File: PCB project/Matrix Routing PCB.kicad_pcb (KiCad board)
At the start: 2 copper layers, 80 x 50.6 mm, 10 parts, among them J1 53261-0471, J2 JST_PH_S4B-PH-SM4-TB, J3 ESQ-105-23-T-D, J4 TSM-102-01-L-DH-A, J5 USB-A-S-X-X-SM2-R, U1 FT232RL

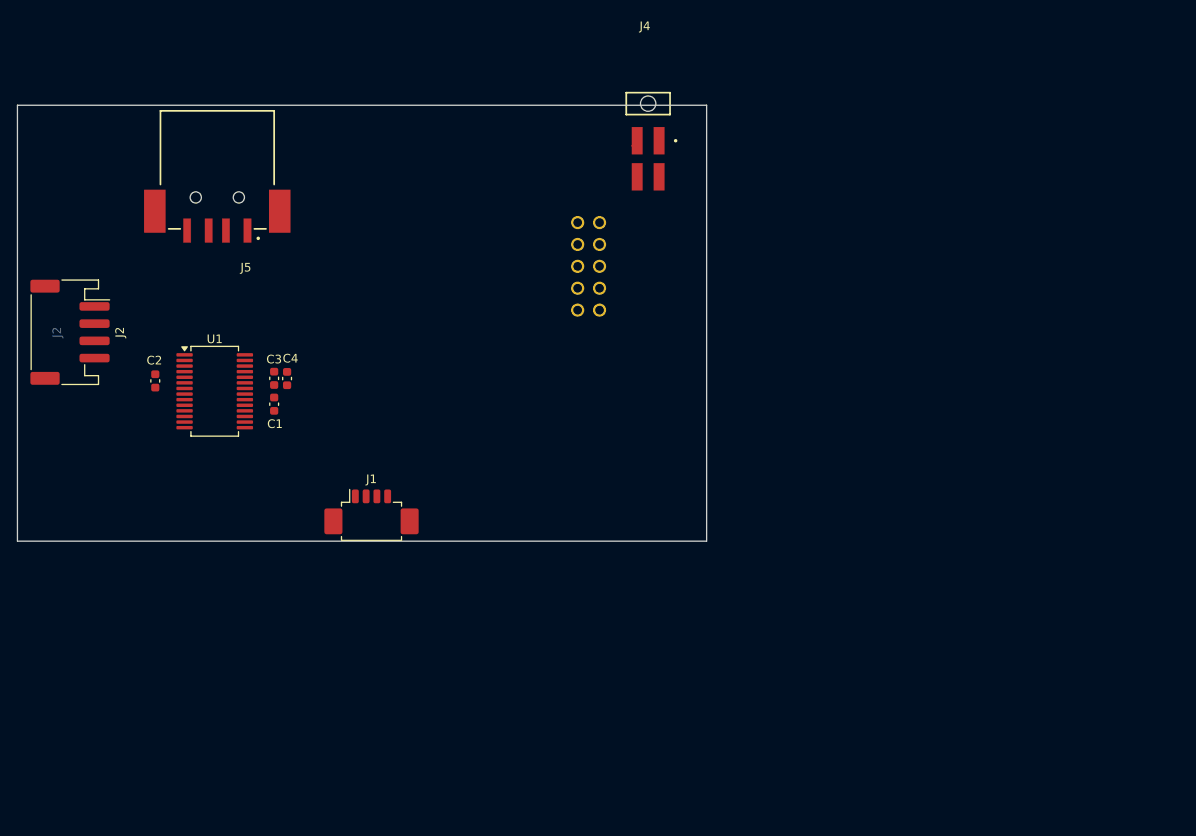
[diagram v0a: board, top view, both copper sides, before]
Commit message: Placement to review
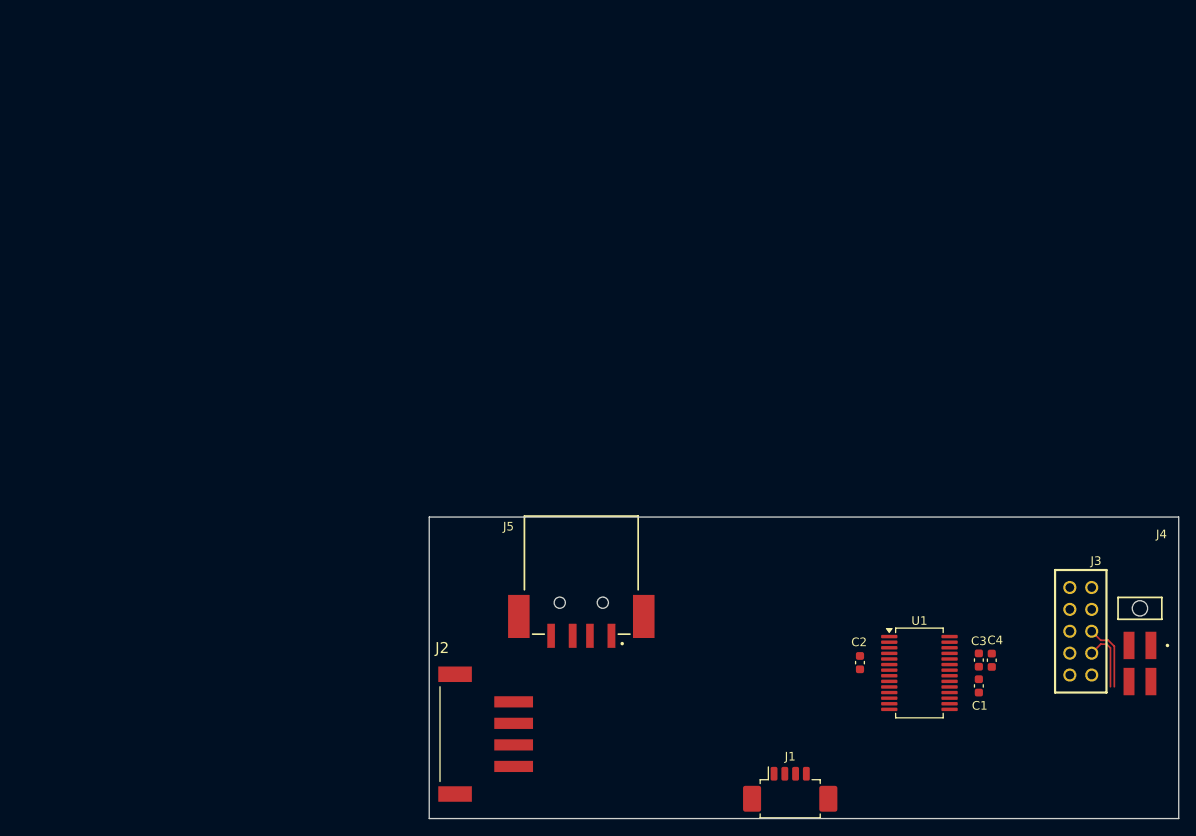
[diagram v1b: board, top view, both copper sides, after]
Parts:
- J2: footprint Matrix Routing PCB:JST_PH_S4B-PH-SM4-TB_1x04-1MP_P2.00mm_Horizontal -> Matrix Routing PCB:S4BXHSM4TBLFSN
- J3: moved to F.Cu
- moved C1 88.1 mm to (172.4, 116.6)
- moved C3 88.1 mm to (172.4, 113.6)
- moved C4 88.1 mm to (173.9, 113.6)
- moved C2 88.1 mm to (158.6, 113.9)
- moved U1 88.1 mm to (165.5, 115.1)
- moved J4 81.8 mm to (191.1, 107.6)
- moved J3 71.1 mm to (184.2, 110.3)
- moved J2 66.4 mm to (114.1, 122.2)
- moved J5 63.2 mm to (126.3, 106.9)
- moved J1 58.3 mm to (150.5, 129.2)
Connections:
- J1 pad 2: /USB2_DN -> /USB1_DN
- J1 pad 3: /USB2_DP -> /USB1_DP
- U1 pad 15: /USB1_DP -> /USB2_DP
- U1 pad 16: /USB1_DN -> /USB2_DN
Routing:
- net /USB1_DP: track 0.00 -> 8.04 mm
- net /USB1_DN: track 0.00 -> 7.30 mm
- net GND: track 0.85 -> 0.00 mm
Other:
- board size 80 x 50.6 mm -> 87 x 35 mm
- board text added: "What is the part number of the device used in the moc pcb"
